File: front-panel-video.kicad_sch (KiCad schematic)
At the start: 0 parts

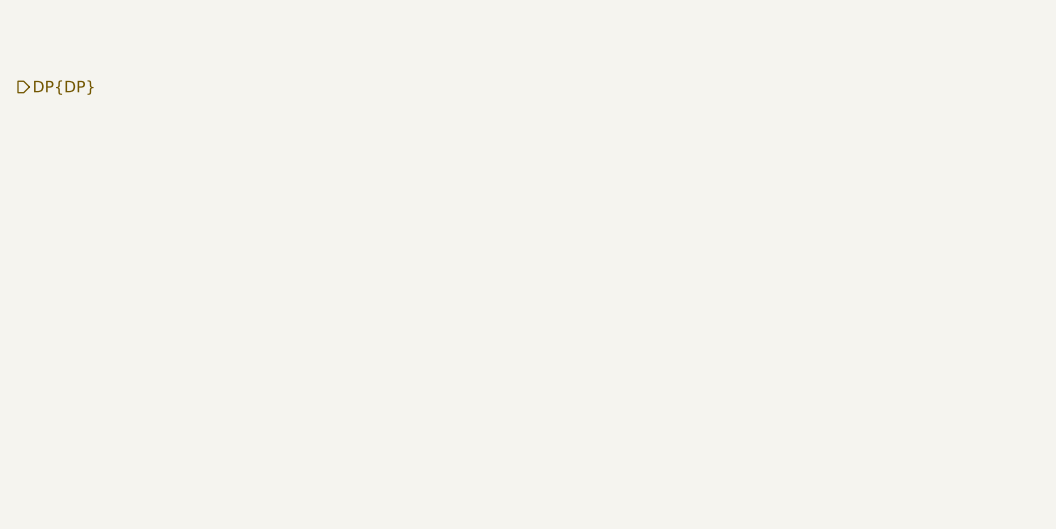
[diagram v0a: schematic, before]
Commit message: [#81876] Add power section
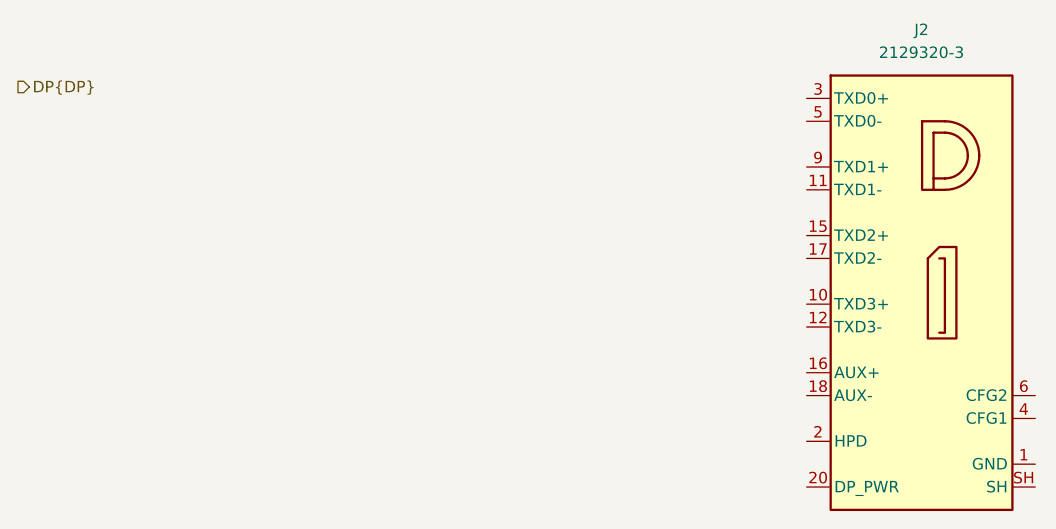
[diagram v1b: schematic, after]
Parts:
- added J2: DisplayPort-Mini_TE_2129320-3, antmicro-footprints:DisplayPort-Mini_Receptacle_TE_2129320-3, symbol antmicroVideoConnectors:DisplayPort-Mini_TE_2129320-3
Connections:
- new net: J2.1 (GND), J2.13 (GND), J2.14 (GND), J2.19 (GND), J2.7 (GND), J2.8 (GND)
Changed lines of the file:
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@@
+		)
+	)
+	(symbol
+		(lib_id "antmicroVideoConnectors:DisplayPort-Mini_TE_2129320-3")
+		(at 153.67 90.17 0)
+		(unit 1)
+		(exclude_from_sim no)
+		(in_bom yes)
+		(on_board yes)
+		(dnp no)
+		(fields_autoplaced yes)
+		(property "Reference" "J2"
+			(at 166.4335 82.55 0)
+			(effects
+				(font
+					(size 1.27 1.27)
+					(thickness 0.15)
+				)
+			)
+		)
+		(property "Value" "DisplayPort-Mini_TE_2129320-3"
+			(at 199.39 90.17 0)
+			(effects
+				(font
+					(size 1.27 1.27)
+					(thickness 0.15)
+				)
+				(justify left bottom)
+				(hide yes)
+			)
+		)
+		(property "Footprint" "antmicro-footprints:DisplayPort-Mini_Receptacle_TE_2129320-3"
+			(at 199.39 92.71 0)
+			(effects
+				(font
+					(size 1.27 1.27)
+					(thickness 0.15)
+				)
+				(justify left bottom)
+				(hide yes)
+			)
+		)
+		(property "Datasheet" "https://www.te.com/usa-en/product-2129320-3.html"
+			(at 199.39 95.25 0)
+			(effects
+				(font
+					(size 1.27 1.27)
+					(thickness 0.15)
+				)
+				(justify left bottom)
+				(hide yes)
+			)
+		)
+		(property "Description" "DisplayPort, Mini Receptacle Connector 20 Position Through Hole, Right Angle"
+			(at 153.67 90.17 0)
+			(effects
+				(font
+					(size 1.27 1.27)
+				)
+				(hide yes)
+			)
+		)
+		(property "MPN" "2129320-3"
+			(at 166.4335 85.09 0)
+			(effects
+				(font
+					(size 1.27 1.27)
+					(thickness 0.15)
+				)
+			)
+		)
+		(property "Manufacturer" "TE Connectivity"
+			(at 199.39 100.33 0)
+			(effects
+				(font
+					(size 1.27 1.27)
+					(thickness 0.15)
+				)
+				(justify left bottom)
+				(hide yes)
+			)
+		)
+		(property "Author" "Antmicro"
+			(at 199.39 102.87 0)
+			(effects
+				(font
+					(size 1.27 1.27)
+					(thickness 0.15)
+				)
+				(justify left bottom)
+				(hide yes)
+			)
+		)
+		(property "License" "Apache-2.0"
+			(at 199.39 105.41 0)
+			(effects
+				(font
+					(size 1.27 1.27)
+					(thickness 0.15)
+				)
+				(justify left bottom)
+				(hide yes)
+			)
+		)
+		(pin "5"
+		)
+		(pin "SH"
+		)
+		(pin "8"
+		)
+		(pin "13"
+		)
+		(pin "19"
+		)
+		(pin "16"
+		)
+		(pin "20"
+		)
+		(pin "15"
+		)
+		(pin "6"
+		)
+		(pin "1"
+		)
+		(pin "11"
+		)
+		(pin "7"
+		)
+		(pin "17"
+		)
+		(pin "14"
+		)
+		(pin "4"
+		)
+		(pin "10"
+		)
+		(pin "2"
+		)
+		(pin "9"
+		)
+		(pin "12"
+		)
+		(pin "18"
+		)
+		(pin "3"
+		)
+		(instances
+			(project ""
+				(path "/5f636c45-3c15-4731-8931-4625e0dab7e4/32de8c9e-be2b-4d78-9d5d-f4e694f2d2e7"
+					(reference "J2")
+					(unit 1)
+				)
+			)
 		)
 	)
